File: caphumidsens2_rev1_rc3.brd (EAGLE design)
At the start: 110 x 10 mm, 12 parts, among them IC1 ATtiny25/45/85/13A

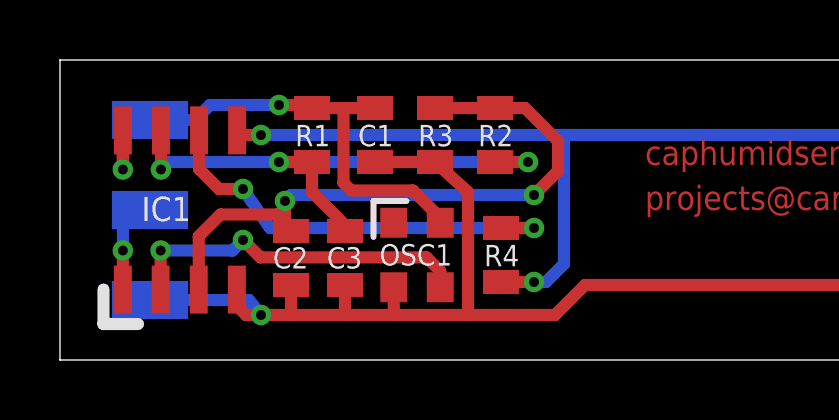
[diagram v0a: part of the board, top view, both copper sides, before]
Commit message: 'improved' routing
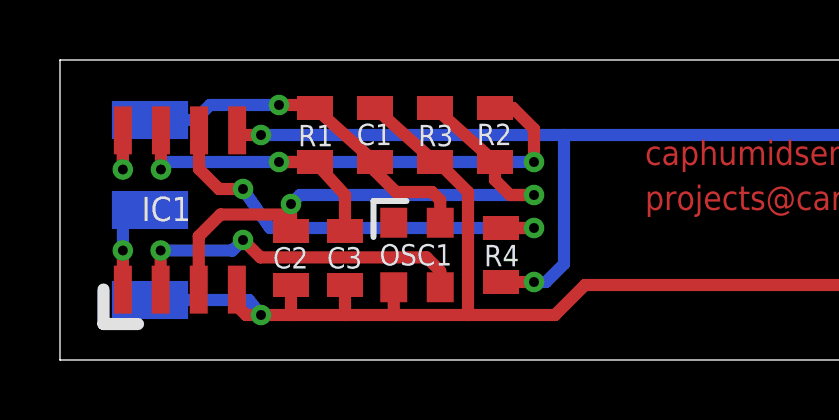
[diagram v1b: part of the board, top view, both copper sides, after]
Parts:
- moved R1 0.10 mm to (8.50, 7.50)
- turned C1 to 270 degrees
- turned R2 to 270 degrees
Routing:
- net 1_3RD_VCC_VREF: track 22.3 -> 20.1 mm
- net 2_3RD_VCC_VREF: track 18.6 -> 20.6 mm
- net VCC: track 17.9 -> 16.0 mm
- net GND: track 46.6 -> 47.4 mm
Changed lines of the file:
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@@
 <attribute name="VALUE" x="4.564" y="1.341" size="0.8128" layer="27" ratio="10" rot="R90"/>
 </element>
-<element name="R2" library="SparkFun" package="0805" value="100k" x="14.5" y="7.5" smashed="yes" rot="R90">
-<attribute name="NAME" x="13.938" y="7.1255" size="0.7112" layer="25" font="vector" ratio="15"/>
-<attribute name="VALUE" x="14.103" y="8.516" size="0.8128" layer="27" rot="R270"/>
+<element name="R2" library="SparkFun" package="0805" value="100k" x="14.5" y="7.5" smashed="yes" rot="R270">
+<attribute name="NAME" x="15.062" y="7.8745" size="0.7112" layer="25" font="vector" ratio="15" rot="R180"/>
+<attribute name="VALUE" x="14.897" y="6.484" size="0.8128" layer="27" rot="R90"/>
 </element>
 <element name="R3" library="SparkFun" package="0805" value="100k" x="12.5" y="7.5" smashed="yes" rot="R90">
@@
 <attribute name="VALUE" x="12.103" y="8.516" size="0.8128" layer="27" rot="R270"/>
 </element>
-<element name="R1" library="SparkFun" package="0805" value="100k" x="8.4" y="7.5" smashed="yes" rot="R270">
-<attribute name="NAME" x="7.838" y="7.1255" size="0.7112" layer="25" font="vector" ratio="15"/>
-<attribute name="VALUE" x="8.003" y="8.516" size="0.8128" layer="27" rot="R270"/>
+<element name="R1" library="SparkFun" package="0805" value="100k" x="8.5" y="7.5" smashed="yes" rot="R270">
+<attribute name="NAME" x="7.938" y="7.1255" size="0.7112" layer="25" font="vector" ratio="15"/>
+<attribute name="VALUE" x="8.103" y="8.516" size="0.8128" layer="27" rot="R270"/>
 </element>
-<element name="C1" library="SparkFun" package="0805" value="100n" x="10.5" y="7.5" smashed="yes" rot="R90">
-<attribute name="NAME" x="9.938" y="7.1255" size="0.7112" layer="25" font="vector" ratio="15"/>
-<attribute name="VALUE" x="10.103" y="8.516" size="0.8128" layer="27" rot="R270"/>
+<element name="C1" library="SparkFun" package="0805" value="100n" x="10.5" y="7.5" smashed="yes" rot="R270">
+<attribute name="NAME" x="11.062" y="7.8745" size="0.7112" layer="25" font="vector" ratio="15" rot="R180"/>
+<attribute name="VALUE" x="10.897" y="6.484" size="0.8128" layer="27" rot="R90"/>
 </element>
 <element name="OSC1" library="seb" package="XO32" value="to be defined" x="11.9" y="3.5" rot="R90"/>
@@
 <wire x1="2.095" y1="7.654" x2="2.095" y2="6.35" width="0.4064" layer="1"/>
 <via x="2.095" y="6.35" extent="1-16" drill="0.3302"/>
-<wire x1="8.4" y1="8.4" x2="9.45" y2="8.4" width="0.4064" layer="1"/>
-<wire x1="8.4" y1="8.4" x2="7.9" y2="8.5" width="0.4064" layer="1"/>
+<wire x1="8.5" y1="8.4" x2="7.9" y2="8.5" width="0.4064" layer="1"/>
 <wire x1="7.9" y1="8.5" x2="7.3" y2="8.5" width="0.4064" layer="1"/>
 <via x="7.3" y="8.5" extent="1-16" drill="0.3302"/>
 <contactref element="OSC1" pad="4"/>
 <contactref element="OSC1" pad="4"/>
-<wire x1="12.675" y1="4.575" x2="12.675" y2="4.7399875" width="0.4064" layer="1"/>
-<wire x1="12.675" y1="4.7399875" x2="11.7649875" y2="5.65" width="0.4064" layer="1"/>
-<wire x1="11.7649875" y1="5.65" x2="9.706153125" y2="5.65" width="0.4064" layer="1"/>
-<wire x1="9.45" y1="5.906153125" x2="9.45" y2="8.4" width="0.4064" layer="1"/>
 <wire x1="3" y1="8" x2="4.5" y2="8" width="0.4064" layer="16"/>
-<wire x1="4.5" y1="8" x2="5" y2="8.5" width="0.4064" layer="16"/>
 <wire x1="5" y1="8.5" x2="7.3" y2="8.5" width="0.4064" layer="16"/>
 <contactref element="C1" pad="2"/>
-<wire x1="9.45" y1="8.4" x2="10.5" y2="8.4" width="0.4064" layer="1"/>
 <wire x1="2.095" y1="6.35" x2="2.095" y2="8" width="0.4064" layer="16"/>
 <wire x1="2.095" y1="8" x2="3" y2="8" width="0.4064" layer="16"/>
-<wire x1="9.45" y1="5.906153125" x2="9.706153125" y2="5.65" width="0.4064" layer="1"/>
+<wire x1="12.675" y1="4.575" x2="12.675" y2="5.325" width="0.4064" layer="1"/>
+<wire x1="12.675" y1="5.325" x2="12.4" y2="5.6" width="0.4064" layer="1"/>
+<wire x1="12.4" y1="5.6" x2="11.2" y2="5.6" width="0.4064" layer="1"/>
+<wire x1="10.4" y1="6.6" x2="10.5" y2="6.6" width="0.4064" layer="1"/>
+<wire x1="10.5" y1="6.6" x2="10.5" y2="6.3" width="0.4064" layer="1"/>
+<wire x1="10.5" y1="6.3" x2="11.2" y2="5.6" width="0.4064" layer="1"/>
+<wire x1="4.5" y1="8" x2="5" y2="8.5" width="0.4064" layer="16"/>
+<wire x1="8.5" y1="8.4" x2="10.5" y2="6.6" width="0.4064" layer="1"/>
 </signal>
 <signal name="GND">
@@
 <contactref element="R3" pad="1"/>
 <contactref element="C1" pad="1"/>
-<wire x1="10.5" y1="6.6" x2="12.5" y2="6.6" width="0.4064" layer="1"/>
 <polygon width="0.4064" layer="1">
 <vertex x="34.5" y="9"/>
@@
 <wire x1="16.5" y1="1.5" x2="17.5" y2="2.5" width="0.4064" layer="1"/>
 <wire x1="17.5" y1="2.5" x2="37" y2="2.5" width="0.4064" layer="1"/>
-<wire x1="12.5" y1="6.6" x2="13.6" y2="5.6" width="0.4064" layer="1"/>
 <wire x1="13.6" y1="5.6" x2="13.6" y2="1.5" width="0.4064" layer="1"/>
 <wire x1="6.2" y1="1.5" x2="6.7" y2="1.5" width="0.4064" layer="1"/>
@@
 <wire x1="7.7" y1="2.5" x2="7.7" y2="1.5" width="0.4064" layer="1"/>
 <wire x1="9.5" y1="2.5" x2="9.5" y2="1.5" width="0.4064" layer="1"/>
+<wire x1="10.5" y1="8.4" x2="12.5" y2="6.6" width="0.4064" layer="1"/>
+<wire x1="12.5" y1="6.6" x2="12.6" y2="6.6" width="0.4064" layer="1"/>
+<wire x1="12.6" y1="6.6" x2="13.6" y2="5.6" width="0.4064" layer="1"/>
 </signal>
 <signal name="2_3RD_VCC_VREF">
@@
 <via x="3.365" y="6.35" extent="1-16" drill="0.3302"/>
 <contactref element="C3" pad="2"/>
-<wire x1="8.4" y1="5.6" x2="9.5" y2="4.5" width="0.4064" layer="1"/>
 <wire x1="9.5" y1="4.5" x2="9.5" y2="4.3" width="0.4064" layer="1"/>
-<wire x1="7.3" y1="6.6" x2="15.6" y2="6.6" width="0.4064" layer="16"/>
-<wire x1="14.5" y1="6.6" x2="15.6" y2="6.6" width="0.4064" layer="1"/>
-<via x="15.6" y="6.6" extent="1-16" drill="0.3302"/>
+<wire x1="7.3" y1="6.6" x2="15.8" y2="6.6" width="0.4064" layer="16"/>
+<via x="15.8" y="6.6" extent="1-16" drill="0.3302"/>
 <via x="7.3" y="6.6" extent="1-16" drill="0.3302"/>
-<wire x1="8.4" y1="5.6" x2="8.4" y2="6.6" width="0.4064" layer="1"/>
-<wire x1="7.3" y1="6.6" x2="8.4" y2="6.6" width="0.4064" layer="1"/>
+<wire x1="7.3" y1="6.6" x2="8.5" y2="6.6" width="0.4064" layer="1"/>
 <wire x1="3.365" y1="6.35" x2="3.615" y2="6.6" width="0.4064" layer="16"/>
 <wire x1="3.615" y1="6.6" x2="7.3" y2="6.6" width="0.4064" layer="16"/>
+<wire x1="14.5" y1="8.4" x2="15.1" y2="8.4" width="0.4064" layer="1"/>
+<wire x1="15.1" y1="8.4" x2="15.8" y2="7.7" width="0.4064" layer="1"/>
+<wire x1="15.8" y1="7.7" x2="15.8" y2="6.6" width="0.4064" layer="1"/>
+<wire x1="8.5" y1="6.6" x2="9.5" y2="5.5" width="0.4064" layer="1"/>
+<wire x1="9.5" y1="5.5" x2="9.5" y2="4.3" width="0.4064" layer="1"/>
 </signal>
 <signal name="1_3RD_VCC_VREF">
 <contactref element="R3" pad="2"/>
 <contactref element="R2" pad="2"/>
-<wire x1="12.5" y1="8.4" x2="14.5" y2="8.4" width="0.4064" layer="1"/>
-<wire x1="14.5" y1="8.4" x2="14.1" y2="8.5" width="0.4064" layer="1"/>
 <contactref element="IC1" pad="3"/>
 <wire x1="4.625" y1="2.346" x2="4.625" y2="2.825" width="0.4064" layer="1"/>
 <contactref element="C2" pad="1"/>
-<wire x1="14.5" y1="8.4" x2="15.5" y2="8.4" width="0.4064" layer="1"/>
 <wire x1="4.625" y1="2.346" x2="4.625" y2="4.125" width="0.4064" layer="1"/>
 <via x="15.8" y="5.5" extent="1-16" drill="0.3302"/>
-<via x="7.5" y="5.3" extent="1-16" drill="0.3302"/>
-<wire x1="15.8" y1="5.5" x2="16.6" y2="6.3" width="0.4064" layer="1"/>
-<wire x1="16.6" y1="6.3" x2="16.6" y2="7.3" width="0.4064" layer="1"/>
-<wire x1="16.6" y1="7.3" x2="15.5" y2="8.4" width="0.4064" layer="1"/>
-<wire x1="7.5" y1="5.3" x2="7.7" y2="5.5" width="0.4064" layer="16"/>
-<wire x1="7.7" y1="5.5" x2="15.8" y2="5.5" width="0.4064" layer="16"/>
+<via x="7.7" y="5.2" extent="1-16" drill="0.3302"/>
 <wire x1="4.625" y1="4.125" x2="5.35" y2="4.85" width="0.4064" layer="1"/>
-<wire x1="5.35" y1="4.85" x2="7.25" y2="4.85" width="0.4064" layer="1"/>
-<wire x1="7.25" y1="4.85" x2="7.5" y2="5" width="0.4064" layer="1"/>
-<wire x1="7.5" y1="5" x2="7.5" y2="5.3" width="0.4064" layer="1"/>
-<wire x1="7.7" y1="4.3" x2="7.5" y2="4.5" width="0.4064" layer="1"/>
-<wire x1="7.5" y1="4.5" x2="7.5" y2="5.3" width="0.4064" layer="1"/>
+<wire x1="14.5" y1="6.6" x2="14.5" y2="6" width="0.4064" layer="1"/>
+<wire x1="14.5" y1="6" x2="15" y2="5.5" width="0.4064" layer="1"/>
+<wire x1="15" y1="5.5" x2="15.8" y2="5.5" width="0.4064" layer="1"/>
+<wire x1="7.7" y1="5.2" x2="8" y2="5.5" width="0.4064" layer="16"/>
+<wire x1="8" y1="5.5" x2="15.8" y2="5.5" width="0.4064" layer="16"/>
+<wire x1="7.7" y1="5.2" x2="7.7" y2="4.3" width="0.4064" layer="1"/>
+<wire x1="5.35" y1="4.85" x2="7.7" y2="4.85" width="0.4064" layer="1"/>
+<wire x1="7.7" y1="4.85" x2="7.7" y2="4.3" width="0.4064" layer="1"/>
+<wire x1="12.5" y1="8.4" x2="14.5" y2="6.6" width="0.4064" layer="1"/>
 </signal>
 <signal name="SENSE_CAP">
